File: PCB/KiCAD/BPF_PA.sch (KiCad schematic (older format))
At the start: 36 parts, among them J4 Conn_Coaxial, J5 Conn_Coaxial, J7 Conn_Coaxial, K1 TQ2-12VDC, Q11 BFG591, Q12 IRF610, Q5 MMBT2222A, T1 1_9, T3 1_4

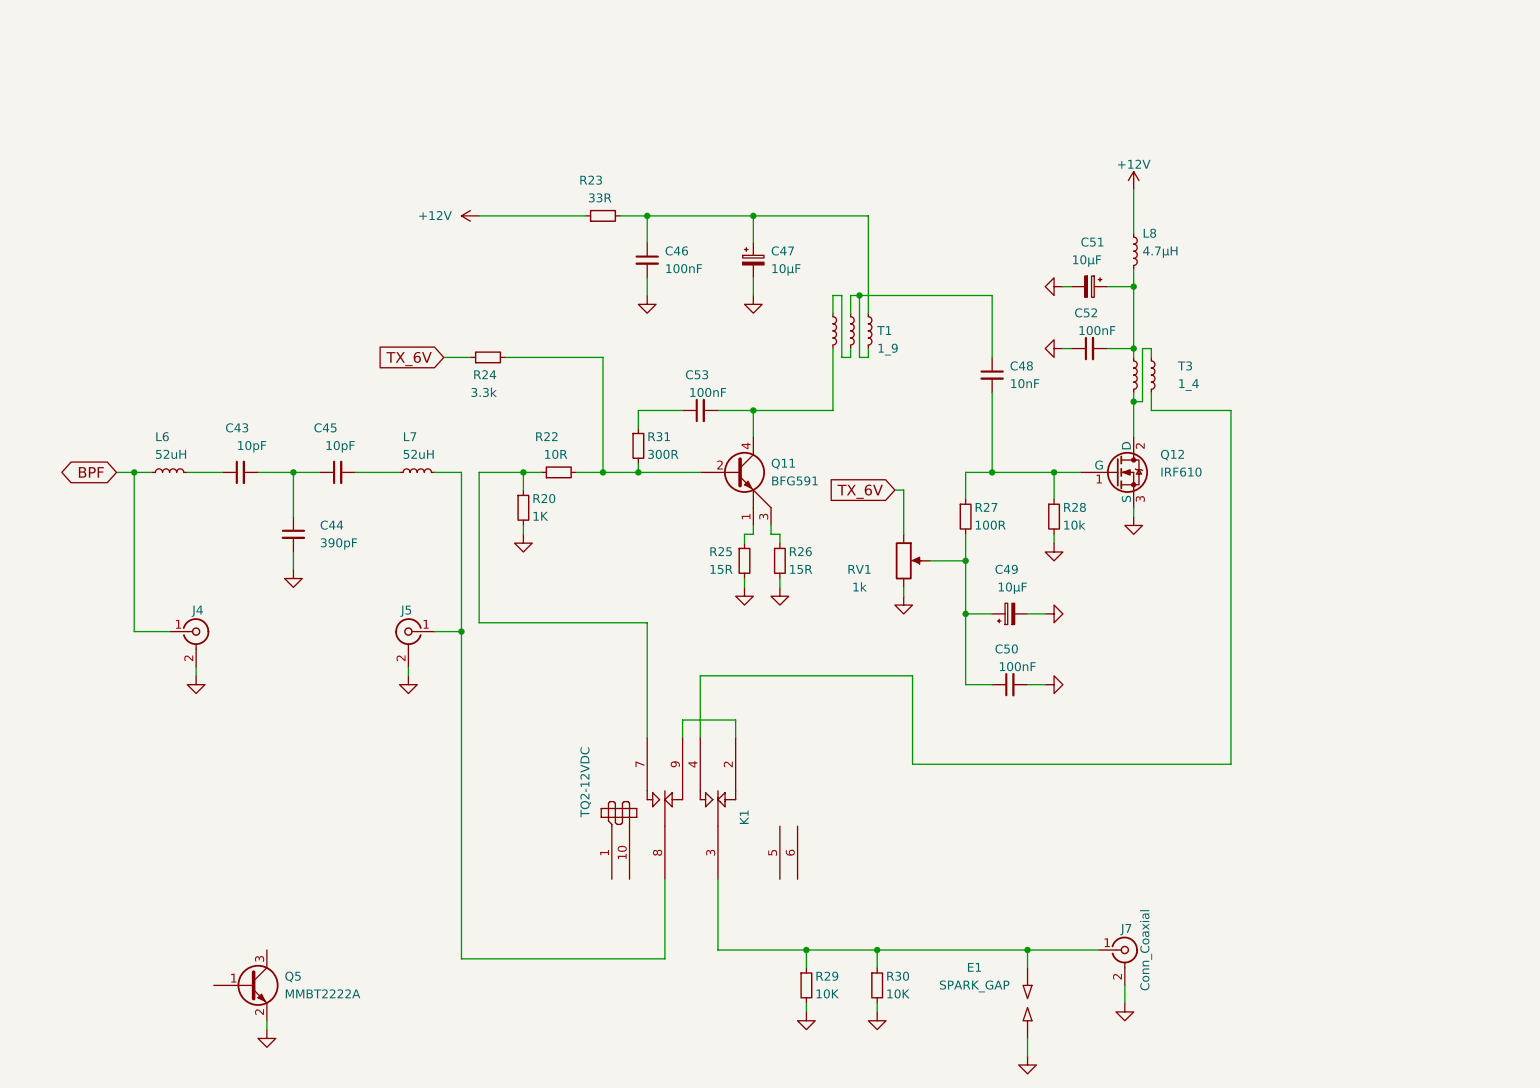
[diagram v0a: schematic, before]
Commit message: PCB home
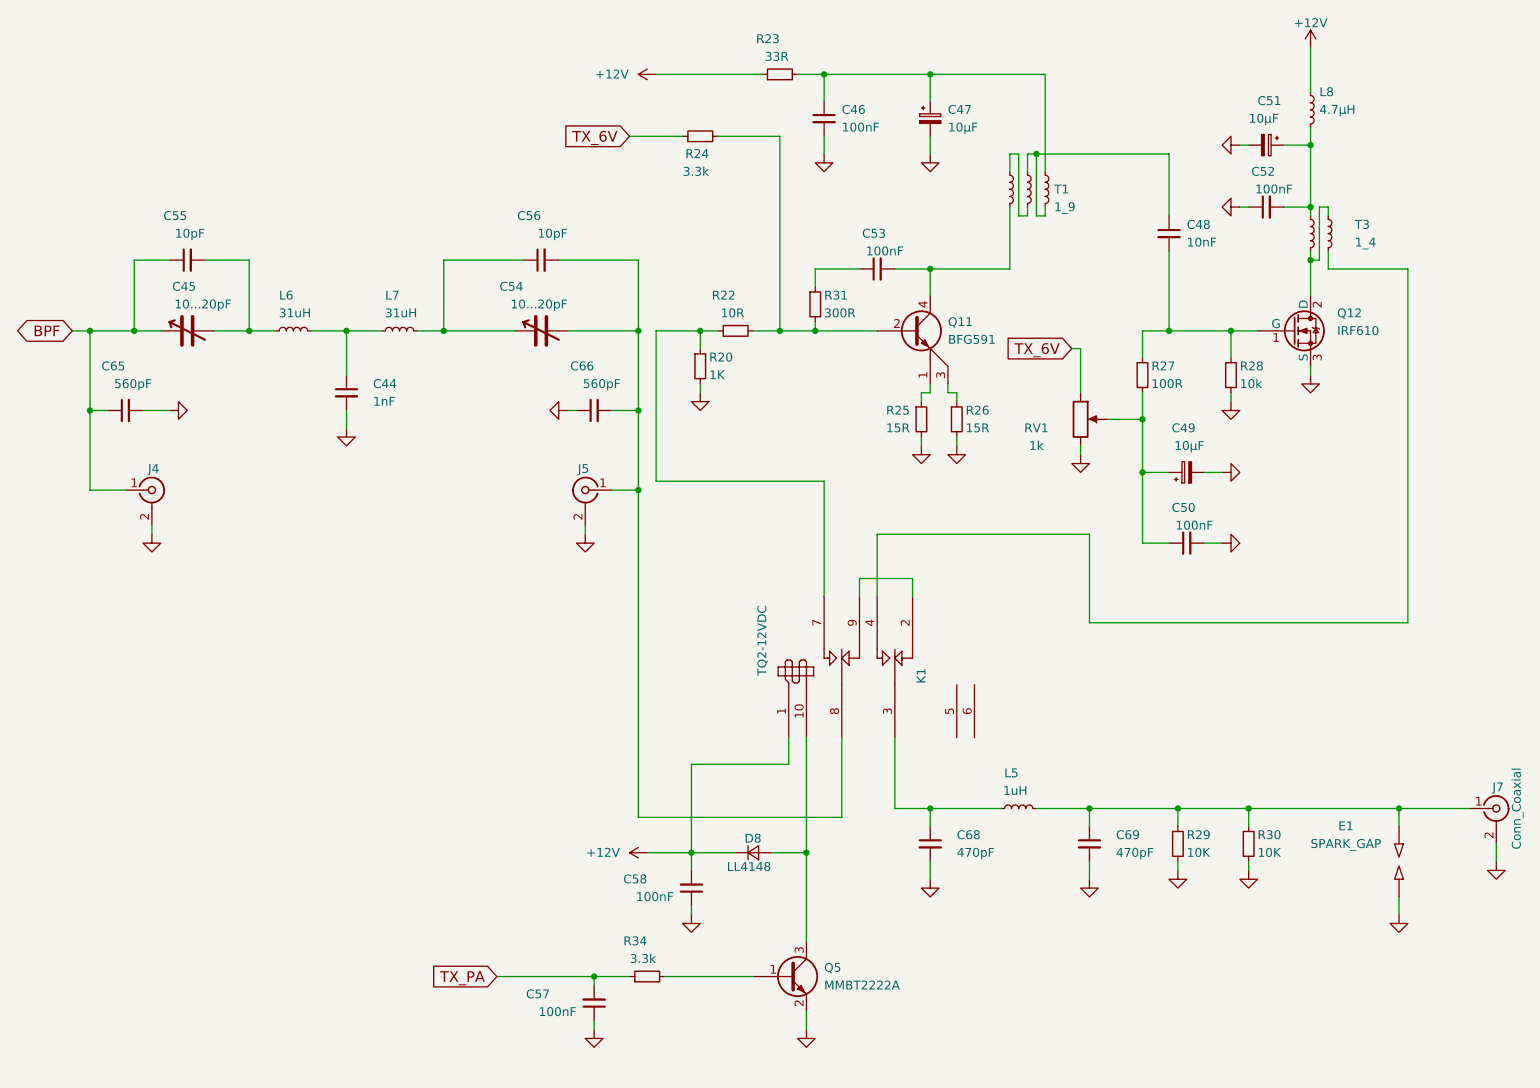
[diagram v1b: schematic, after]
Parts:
- removed C43, C45: 10pF, DragonFly:C_1206_0603, symbol C_Small
- added C45, C54: 10...20pF, Capacitors_SMD:C_Trimmer_Voltronics_JZ, symbol C_Variable
- added C55, C56: 10pF, DragonFly:C_1206_0603, symbol C_Small
- added C57, C58: 100nF, Capacitors_SMD:C_0603_HandSoldering, symbol C_Small
- added C65, C66: 560pF, DragonFly:C_1206_0603, symbol C_Small
- added C68, C69: 470pF, Capacitors_THT:C_Disc_D6.0mm_W2.5mm_P5.00mm, symbol C_Small
- added D8: LL4148, Diodes_SMD:D_MiniMELF, symbol D_Small
- added L5: 1uH, Resistors_THT:R_Axial_DIN0411_L9.9mm_D3.6mm_P12.70mm_Horizontal, symbol L_Small
- added R34: 3.3k, DragonFly:R_1206_0603, symbol R_Small
- C44: value 390pF -> 1nF
- J4, J5: footprint (none) -> DragonFly:U.FL_Molex_MCRF_73412-0110_Vertical
- L6, L7: value 52uH -> 31uH; footprint (none) -> Choke_Toroid_ThroughHole:Choke_Toroid_5x10mm_Vertical
- R29, R30: footprint (none) -> DragonFly:R_1206_0603
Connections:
- net +12V: now also K1.1 (+), C58.2, D8.1 (K)
- net BPF: now also C45.1, C55.1, C65.1; no longer L6.1
- net GND: now also C57.1, C58.1, C65.2, C66.1, C68.2, C69.2
- net at L6.2: now also C44.1, L7.1
- net at J5.1 (In), K1.8 (C1): now also C54.2, C56.2, C66.2; no longer L7.2
- net at K1.10 (-): now also Q5.3 (C), D8.2 (A)
- net at E1.1, J7.1 (In), R29.1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: now also C69.1, L5.2; no longer K1.3 (C2)
- net at Q5.1 (B): now also R34.2
- new net: C45.2, C55.2, L6.1
- new net: C54.1, C56.1, L7.2
- new net: C68.1, K1.3 (C2), L5.1
- new net TX_PA: C57.2, R34.1
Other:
- moved on the sheet: C44, C46, C47, C48, C49, C50, C51, C52, C53, E1, J4, J5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
